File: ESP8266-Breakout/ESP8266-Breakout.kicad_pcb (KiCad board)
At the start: 2 copper layers, 26.2 x 40 mm, 23 parts, among them J101 Conn_01x08_Female, J102 Conn_01x08_Female, J103 FTDI, SW101 Flash, SW102 RST, U102 ESP-12F

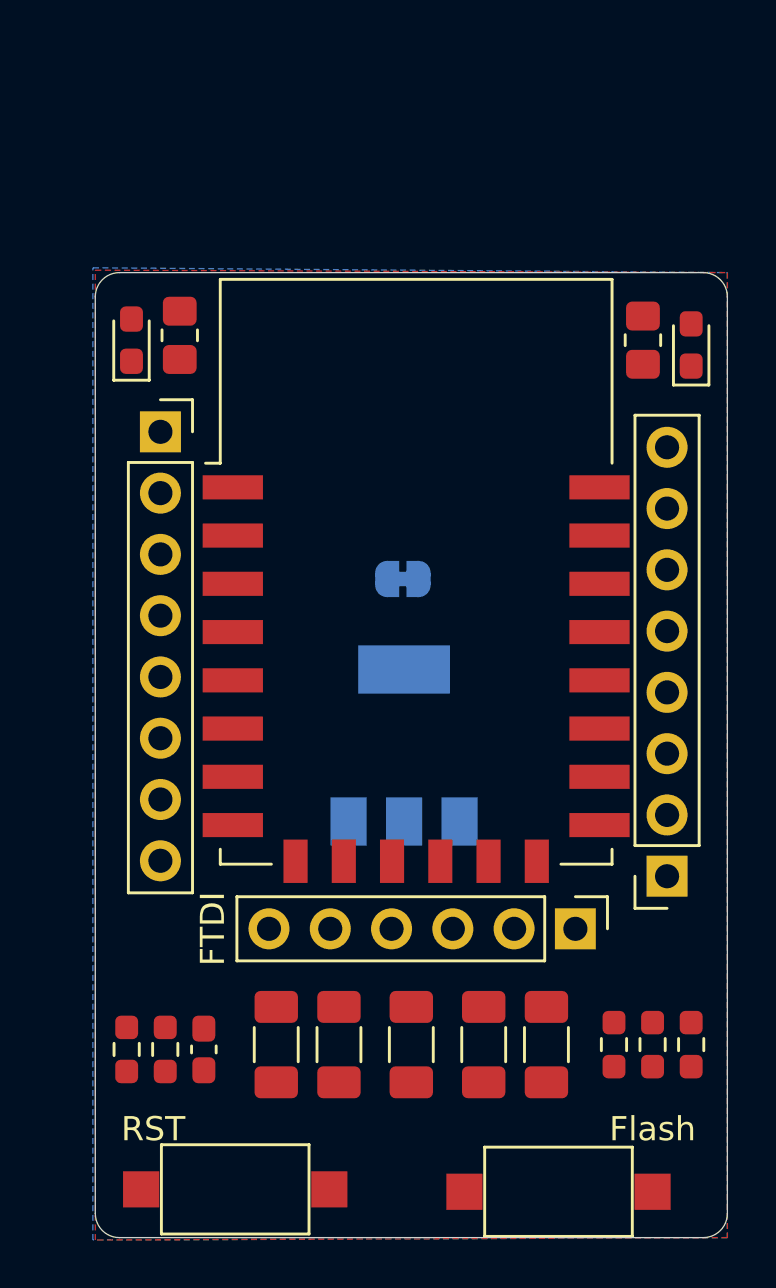
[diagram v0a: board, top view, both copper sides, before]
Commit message: New version completed, shematic + pcb wired
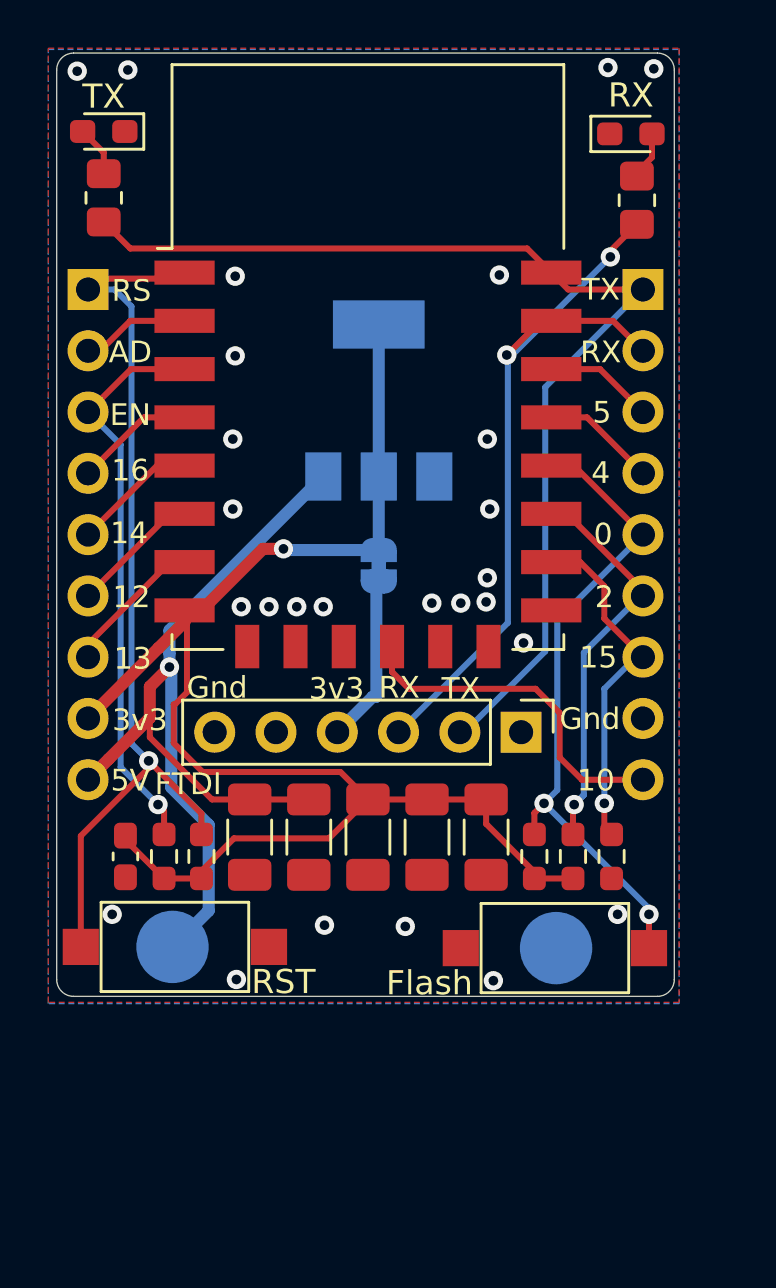
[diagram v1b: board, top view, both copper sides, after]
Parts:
- removed C105: 100nF, Capacitor_SMD:C_1206_3216Metric_Pad1.33x1.80mm_HandSolder
- removed C106: 10uF, Capacitor_SMD:C_1206_3216Metric_Pad1.33x1.80mm_HandSolder
- removed D101: TX, LED_SMD:LED_0603_1608Metric_Pad1.05x0.95mm_HandSolder
- removed D102: RX, LED_SMD:LED_0603_1608Metric_Pad1.05x0.95mm_HandSolder
- removed J103: FTDI, Connector_PinHeader_2.54mm:PinHeader_1x06_P2.54mm_Vertical
- removed JP101: Power, Jumper:SolderJumper-2_P1.3mm_Bridged_RoundedPad1.0x1.5mm
- removed R101, R102, R103, R105, R106: 10K, Resistor_SMD:R_0603_1608Metric_Pad0.98x0.95mm_HandSolder
- removed R104, R107: 15, Resistor_SMD:R_0805_2012Metric_Pad1.20x1.40mm_HandSolder
- removed SW101: Flash, Button_Switch_SMD:SW_SPST_CK_RS282G05A3
- removed SW102: RST, Button_Switch_SMD:SW_SPST_CK_RS282G05A3
- removed U102: ESP-12F, RF_Module:ESP-12E
- removed Ue: AMS1117-3.3, Package_TO_SOT_SMD:SOT-223-3_TabPin2
- added C501: 0.1uF, Capacitor_SMD:C_0603_1608Metric_Pad1.08x0.95mm_HandSolder, F.Cu at (142.2, 98.4)
- added C502: 47uF, Capacitor_SMD:C_1206_3216Metric_Pad1.33x1.80mm_HandSolder, F.Cu at (152.2, 97.6)
- added D501: TX, LED_SMD:LED_0603_1608Metric_Pad1.05x0.95mm_HandSolder, F.Cu at (141.2, 68.3)
- added D502: RX, LED_SMD:LED_0603_1608Metric_Pad1.05x0.95mm_HandSolder, F.Cu at (163.1, 68.5)
- added J501: FTDI, Connector_PinHeader_2.54mm:PinHeader_1x06_P2.54mm_Vertical, F.Cu at (158.6, 93.2)
- added JP501: Power, Jumper:SolderJumper-2_P1.3mm_Bridged_RoundedPad1.0x1.5mm, B.Cu at (152.7, 86.3)
- added R501: 10K, Resistor_SMD:R_0603_1608Metric_Pad0.98x0.95mm_HandSolder, F.Cu at (159.1, 98.4)
- added R502: 10K, Resistor_SMD:R_0603_1608Metric_Pad0.98x0.95mm_HandSolder, F.Cu at (145.3, 98.4)
- added R503: 10K, Resistor_SMD:R_0603_1608Metric_Pad0.98x0.95mm_HandSolder, F.Cu at (143.8, 98.4)
- added R504: 15, Resistor_SMD:R_0805_2012Metric_Pad1.20x1.40mm_HandSolder, F.Cu at (141.2, 71.1)
- added R505: 10K, Resistor_SMD:R_0603_1608Metric_Pad0.98x0.95mm_HandSolder, F.Cu at (160.7, 98.4)
- added R506: 10K, Resistor_SMD:R_0603_1608Metric_Pad0.98x0.95mm_HandSolder, F.Cu at (162.3, 98.4)
- added R507: 15, Resistor_SMD:R_0805_2012Metric_Pad1.20x1.40mm_HandSolder, F.Cu at (163.3, 71.2)
- added SW501: Flash, Button_Switch_SMD:SW_SPST_CK_RS282G05A3, F.Cu at (159.9, 102.2)
- added SW502: RST, Button_Switch_SMD:SW_SPST_CK_RS282G05A3, F.Cu at (144.2, 102.2)
- added TP101: TestPoint, TestPoint:TestPoint_Pad_D3.0mm, B.Cu at (144.1, 102.2)
- added TP102: TestPoint, TestPoint:TestPoint_Pad_D3.0mm, B.Cu at (160.0, 102.2)
- added U101: AMS1117-3.3, Package_TO_SOT_SMD:SOT-223-3_TabPin2, B.Cu at (152.7, 79.5)
- added U501: ESP-12F, RF_Module:ESP-12E, F.Cu at (152.2, 77.7)
- C102: value 0.1uF -> 100nF; footprint Capacitor_SMD:C_0603_1608Metric_Pad1.08x0.95mm_HandSolder -> Capacitor_SMD:C_1206_3216Metric_Pad1.33x1.80mm_HandSolder
- C104: value 47uF -> 10uF
- J101, J102: value Conn_01x08_Female -> Conn_01x09_Female; footprint Connector_PinSocket_2.54mm:PinSocket_1x08_P2.54mm_Vertical -> Custom:PinHeader_1x09_P2.54mm_Vertical_without_silkscrean
- moved J102 24.3 mm to (163.6, 74.9), turned to 0 degrees
- moved C103 9.34 mm to (154.7, 97.6)
- moved C104 9.14 mm to (157.1, 97.6)
- moved C102 9.00 mm to (147.3, 97.6), turned to 270 degrees
- moved C101 8.71 mm to (149.8, 97.6)
- moved J101 6.62 mm to (140.6, 74.9)
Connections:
- C102 pad 1: +3V3 -> +5V
- C103 pad 1: +5V -> +3V3
- J101 pad 1: /~RST -> /RST
- J102 pad 1: GND -> /GPIO1
- J102 pad 2: /GPIO15 -> /GPIO3
- J102 pad 3: /GPIO2 -> /GPIO5
- J102 pad 4: /~FLASH -> /GPIO4
- J102 pad 5: /GPIO4 -> /GPIO0
- J102 pad 6: /GPIO5 -> /GPIO2
- J102 pad 7: /RX -> /GPIO15
- J102 pad 8: /TX -> GND
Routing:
- net +3V3: track 0.00 -> 62.5 mm, vias 0 -> 1
- net /GPIO1: track 0.00 -> 45.1 mm
- net +5V: track 0.00 -> 41.4 mm, vias 0 -> 1
- net /RST: track 0.00 -> 38.6 mm, vias 0 -> 1
- net /GPIO3: track 0.00 -> 32.1 mm, vias 0 -> 2
- net /GPIO0: track 0.00 -> 27.1 mm, vias 0 -> 2
- net /EN: track 0.00 -> 23.5 mm, vias 0 -> 1
- net /GPIO2: track 0.00 -> 16.9 mm, vias 0 -> 1
- net /GPIO15: track 0.00 -> 14.5 mm, vias 0 -> 1
- net /GPIO10: track 0.00 -> 14.4 mm
- net Net-(J501-Pad4): track 0.00 -> 7.05 mm
- net /GPIO13: track 0.00 -> 5.95 mm
- net /GPIO12: track 0.00 -> 5.41 mm
- net /GPIO14: track 0.00 -> 5.18 mm
- net /GPIO16: track 0.00 -> 4.96 mm
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- added copper zone on B.Cu, net GND
- removed copper zone on B.Cu, net (none)
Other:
- board size 26.2 x 40 mm -> 25.6 x 39.1 mm
- board text added: "0"
- board text added: "10"
- board text added: "12"
- board text added: "13"
- board text added: "14"
- board text added: "15"
- board text added: "16"
- board text added: "2"
- board text added: "3v3"
- board text added: "4"
- board text added: "5"
- board text added: "5V"
- board text added: "AD"
- board text added: "EN"
- board text added: "Gnd"
- board text added: "RS"
- board text added: "RX"
- board text added: "TX"
